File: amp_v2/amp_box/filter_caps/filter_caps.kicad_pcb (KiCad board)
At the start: 2 copper layers, 90.2 x 50.8 mm, 20 parts, among them P1 CONN_2, P2 CONN_2, P3 CONN_2, P4 CONN_2, P5 CONN_2, P6 CONN_2

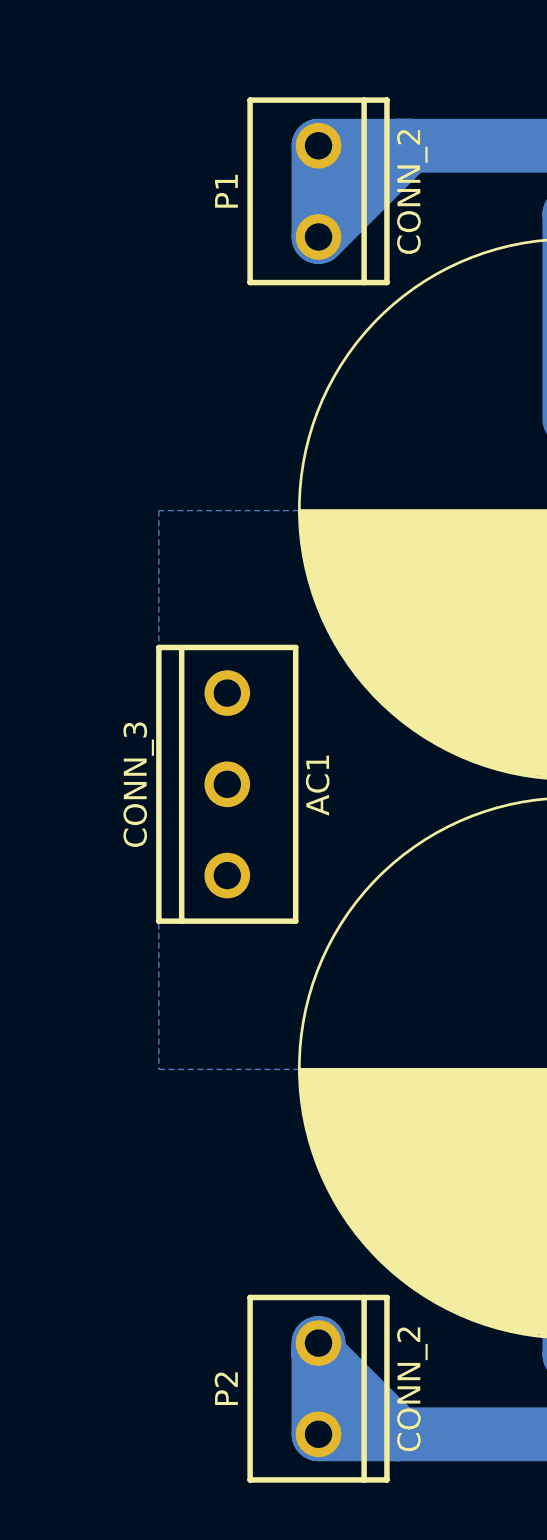
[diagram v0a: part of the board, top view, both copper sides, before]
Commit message: updates
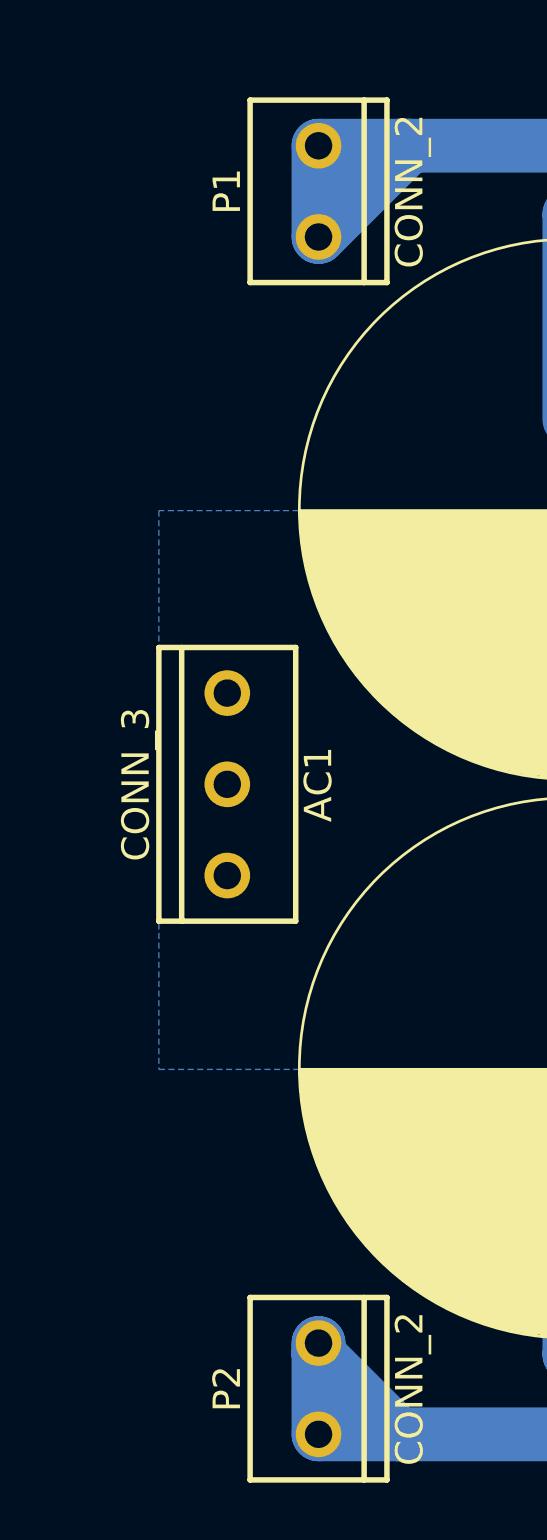
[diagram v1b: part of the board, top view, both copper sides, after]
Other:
- net class Default removed
